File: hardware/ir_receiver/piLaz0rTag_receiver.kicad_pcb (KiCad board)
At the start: 2 copper layers, 56.9 x 27.9 mm, 4 parts, among them U1 TSOP4838

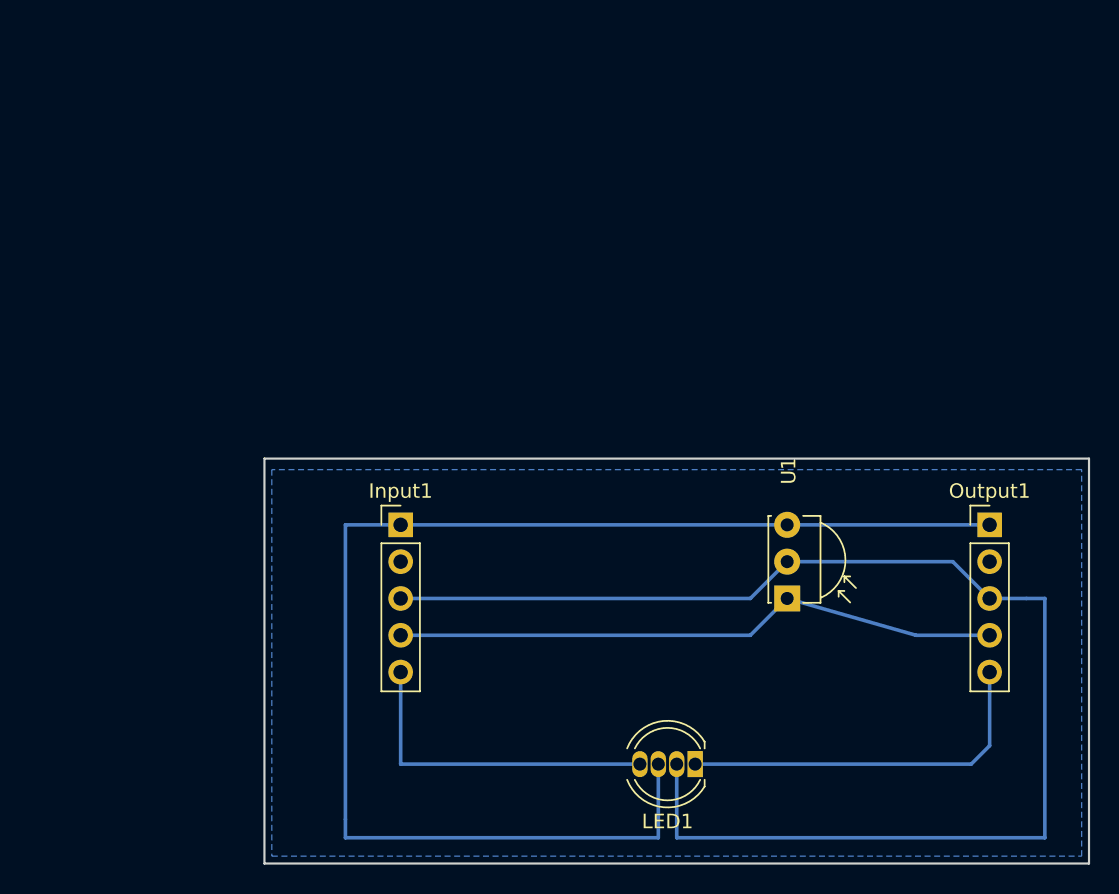
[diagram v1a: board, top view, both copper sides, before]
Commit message: #9 Add gerber files
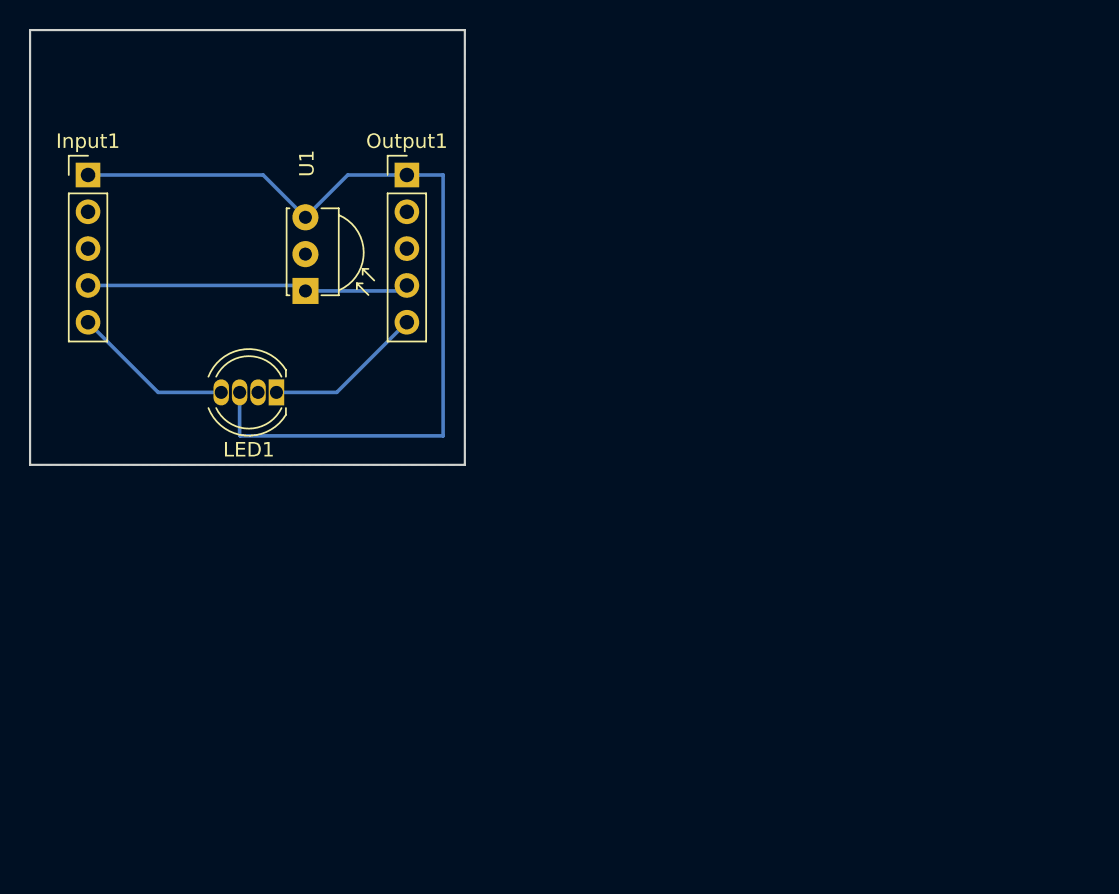
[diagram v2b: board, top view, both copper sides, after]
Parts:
- moved Output1 46.9 mm to (116.0, 80.0)
- moved U1 39.4 mm to (109.0, 88.0)
- moved LED1 38.6 mm to (107.0, 95.0)
- moved Input1 32.4 mm to (94.0, 80.0)
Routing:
- net Net-(Input1-Pad3): track 93.5 -> 0.00 mm
- net Net-(Input1-Pad1): track 92.7 -> 61.9 mm
- net Net-(Input1-Pad4): track 42.0 -> 22.3 mm
- net Net-(LED1-Pad1): track 25.9 -> 11.0 mm
- net Net-(Input1-Pad5): track 22.9 -> 11.2 mm
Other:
- board size 56.9 x 27.9 mm -> 30 x 30 mm
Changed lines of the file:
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@@
     (links 10)
     (no_connects 0)
-    (area 106.096999 99.492999 163.143001 127.583001)
+    (area 89.924999 69.924999 120.075001 100.075001)
     (thickness 1.6)
     (drawings 4)
-    (tracks 25)
+    (tracks 17)
     (zones 0)
     (modules 4)
@@
   )
   (module Socket_Strips:Socket_Strip_Straight_1x05_Pitch2.54mm (layer F.Cu)
-    (at 115.57 104.14)
+    (at 94 80)
     (descr "Through hole straight socket strip, 1x05, 2.54mm pitch, single row")
     (tags "Through hole socket strip THT 1x05 2.54mm single row")
@@
   )
   (module LEDs:LED_D5.0mm-4 (layer F.Cu)
-    (at 135.89 120.65 180)
+    (at 107 95 180)
     (descr "LED, diameter 5.0mm, 2 pins, diameter 5.0mm, 3 pins, diameter 5.0mm, 4 pins, http://www.kingbright.com/attachments/file/psearch/000/00/00/L-154A4SUREQBFZGEW(Ver.9A).pdf")
     (tags "LED diameter 5.0mm 2 pins diameter 5.0mm 3 pins diameter 5.0mm 4 pins")
@@
   )
   (module Socket_Strips:Socket_Strip_Straight_1x05_Pitch2.54mm (layer F.Cu)
-    (at 156.21 104.14)
+    (at 116 80)
     (descr "Through hole straight socket strip, 1x05, 2.54mm pitch, single row")
     (tags "Through hole socket strip THT 1x05 2.54mm single row")
@@
   )
   (module Opto-Devices:IRReceiver_Vishay_MOLD-3pin (layer F.Cu)
-    (at 142.24 109.22 90)
+    (at 109 88 90)
     (descr "IR Receiver Vishay TSOP-xxxx, MOLD package")
     (tags "IR Receiver Vishay TSOP-xxxx MOLD")
@@
       (net 1 "Net-(Input1-Pad1)"))
   )
-  (gr_line (start 106.172 99.568) (end 163.068 99.568) (angle 90) (layer Edge.Cuts) (width 0.15))
-  (gr_line (start 106.172 127.508) (end 106.172 99.568) (angle 90) (layer Edge.Cuts) (width 0.15))
-  (gr_line (start 163.068 127.508) (end 106.172 127.508) (angle 90) (layer Edge.Cuts) (width 0.15))
-  (gr_line (start 163.068 99.568) (end 163.068 127.508) (angle 90) (layer Edge.Cuts) (width 0.15))
-  (segment (start 115.57 104.14) (end 111.76 104.14) (width 0.25) (layer B.Cu) (net 1))
-  (segment (start 133.35 125.73) (end 133.35 120.65) (width 0.25) (layer B.Cu) (net 1))
-  (segment (start 111.76 125.73) (end 133.35 125.73) (width 0.25) (layer B.Cu) (net 1))
-  (segment (start 111.76 124.46) (end 111.76 125.73) (width 0.25) (layer B.Cu) (net 1))
-  (segment (start 111.76 104.14) (end 111.76 124.46) (width 0.25) (layer B.Cu) (net 1))
-  (segment (start 115.57 104.14) (end 142.24 104.14) (width 0.25) (layer B.Cu) (net 1))
-  (segment (start 142.24 104.14) (end 156.21 104.14) (width 0.25) (layer B.Cu) (net 1))
-  (segment (start 156.21 109.22) (end 158.75 109.22) (width 0.25) (layer B.Cu) (net 3))
-  (segment (start 134.62 125.73) (end 134.62 120.65) (width 0.25) (layer B.Cu) (net 3))
-  (segment (start 160.02 125.73) (end 134.62 125.73) (width 0.25) (layer B.Cu) (net 3))
-  (segment (start 160.02 109.22) (end 160.02 125.73) (width 0.25) (layer B.Cu) (net 3))
-  (segment (start 158.75 109.22) (end 160.02 109.22) (width 0.25) (layer B.Cu) (net 3))
-  (segment (start 115.57 109.22) (end 139.7 109.22) (width 0.25) (layer B.Cu) (net 3))
-  (segment (start 139.7 109.22) (end 142.24 106.68) (width 0.25) (layer B.Cu) (net 3))
-  (segment (start 142.24 106.68) (end 153.67 106.68) (width 0.25) (layer B.Cu) (net 3))
-  (segment (start 153.67 106.68) (end 156.21 109.22) (width 0.25) (layer B.Cu) (net 3))
-  (segment (start 142.24 109.22) (end 151.13 111.76) (width 0.25) (layer B.Cu) (net 4))
-  (segment (start 151.13 111.76) (end 156.21 111.76) (width 0.25) (layer B.Cu) (net 4))
-  (segment (start 115.57 111.76) (end 139.7 111.76) (width 0.25) (layer B.Cu) (net 4))
-  (segment (start 139.7 111.76) (end 142.24 109.22) (width 0.25) (layer B.Cu) (net 4))
-  (segment (start 115.57 114.3) (end 115.57 120.65) (width 0.25) (layer B.Cu) (net 5))
-  (segment (start 115.57 120.65) (end 132.08 120.65) (width 0.25) (layer B.Cu) (net 5))
-  (segment (start 135.89 120.65) (end 154.94 120.65) (width 0.25) (layer B.Cu) (net 7))
-  (segment (start 156.21 119.38) (end 156.21 114.3) (width 0.25) (layer B.Cu) (net 7))
-  (segment (start 154.94 120.65) (end 156.21 119.38) (width 0.25) (layer B.Cu) (net 7))
+  (gr_line (start 120 100) (end 90 100) (angle 90) (layer Edge.Cuts) (width 0.15))
+  (gr_line (start 120 70) (end 120 100) (angle 90) (layer Edge.Cuts) (width 0.15))
+  (gr_line (start 90 70) (end 120 70) (angle 90) (layer Edge.Cuts) (width 0.15))
+  (gr_line (start 90 100) (end 90 70) (angle 90) (layer Edge.Cuts) (width 0.15))
+  (segment (start 104.46 95) (end 104.46 97.96) (width 0.25) (layer B.Cu) (net 1) (status 400000))
+  (segment (start 118.5 80) (end 116 80) (width 0.25) (layer B.Cu) (net 1) (status 800000))
+  (segment (start 118.5 98) (end 118.5 80) (width 0.25) (layer B.Cu) (net 1))
+  (segment (start 104.5 98) (end 118.5 98) (width 0.25) (layer B.Cu) (net 1))
+  (segment (start 104.46 97.96) (end 104.5 98) (width 0.25) (layer B.Cu) (net 1))
+  (segment (start 116 80) (end 111.92 80) (width 0.25) (layer B.Cu) (net 1))
+  (segment (start 111.92 80) (end 109 82.92) (width 0.25) (layer B.Cu) (net 1))
+  (segment (start 94 80) (end 106.08 80) (width 0.25) (layer B.Cu) (net 1))
+  (segment (start 106.08 80) (end 109 82.92) (width 0.25) (layer B.Cu) (net 1))
+  (segment (start 109 88) (end 115.62 88) (width 0.25) (layer B.Cu) (net 4))
+  (segment (start 115.62 88) (end 116 87.62) (width 0.25) (layer B.Cu) (net 4))
+  (segment (start 94 87.62) (end 108.62 87.62) (width 0.25) (layer B.Cu) (net 4))
+  (segment (start 108.62 87.62) (end 109 88) (width 0.25) (layer B.Cu) (net 4))
+  (segment (start 103.19 95) (end 98.84 95) (width 0.25) (layer B.Cu) (net 5))
+  (segment (start 98.84 95) (end 94 90.16) (width 0.25) (layer B.Cu) (net 5))
+  (segment (start 107 95) (end 111.16 95) (width 0.25) (layer B.Cu) (net 7))
+  (segment (start 111.16 95) (end 116 90.16) (width 0.25) (layer B.Cu) (net 7))
   (zone (net 3) (net_name "Net-(Input1-Pad3)") (layer B.Cu) (hatch edge 0.508)
     (connect_pads (clearance 0.508))
@@
     (polygon
       (pts
-        (xy 106.68 100.33) (xy 106.68 127) (xy 162.56 127) (xy 162.56 100.33)
+        (xy 90 70) (xy 120 70) (xy 120 100) (xy 90 100)
       )
     )
